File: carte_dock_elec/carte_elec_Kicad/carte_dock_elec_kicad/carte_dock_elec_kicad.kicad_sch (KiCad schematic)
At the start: 13 parts, among them J1 1758018, J10 Conn_02x20_Odd_Even, J2 22053021, J3 22272041, J4 22272041, J5 22272041, J6 1758018, J7 1758018, J8 1758018, J9 1758018, Q1 IRLB8748PBF

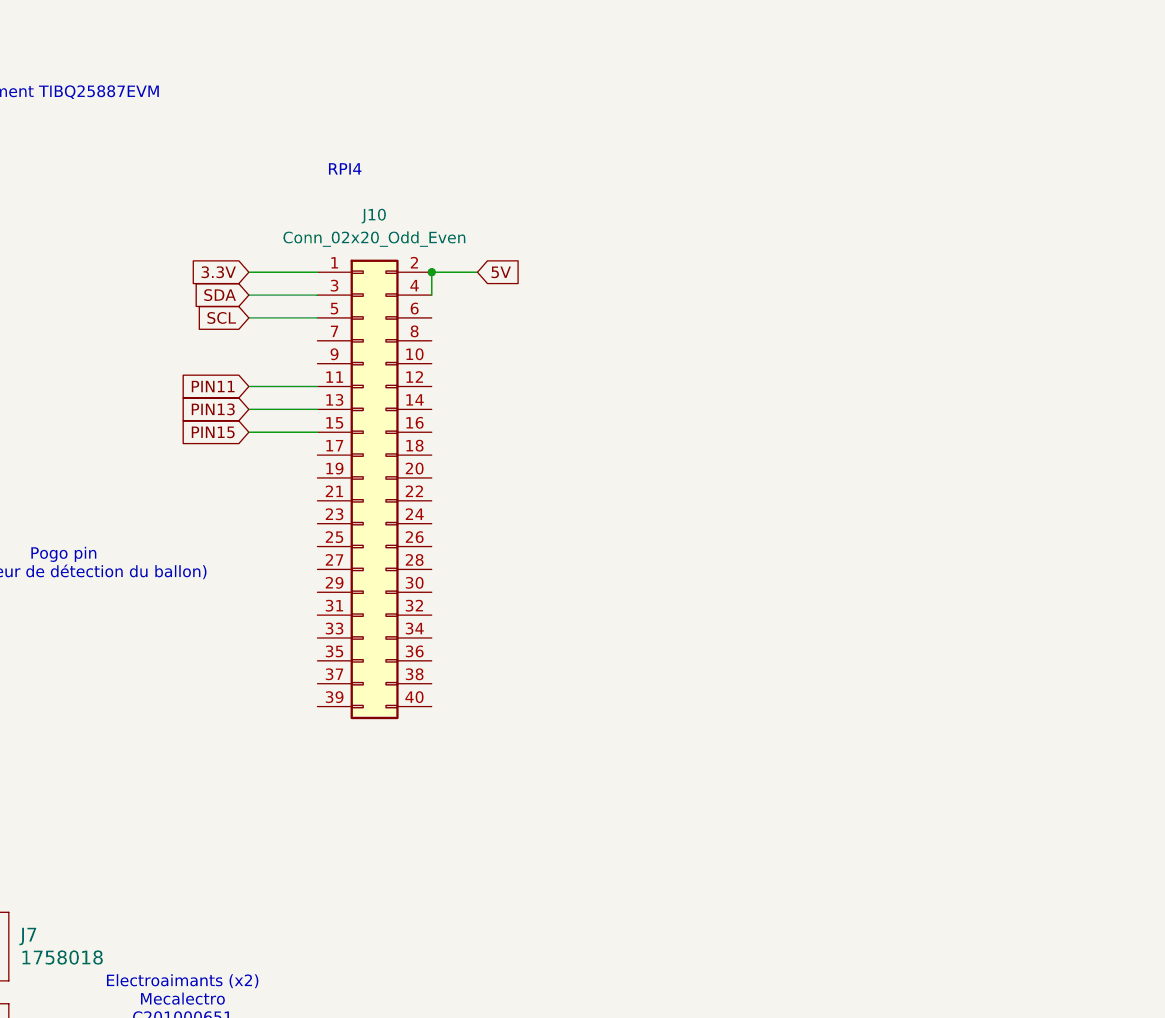
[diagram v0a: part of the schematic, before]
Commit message: carte_dock
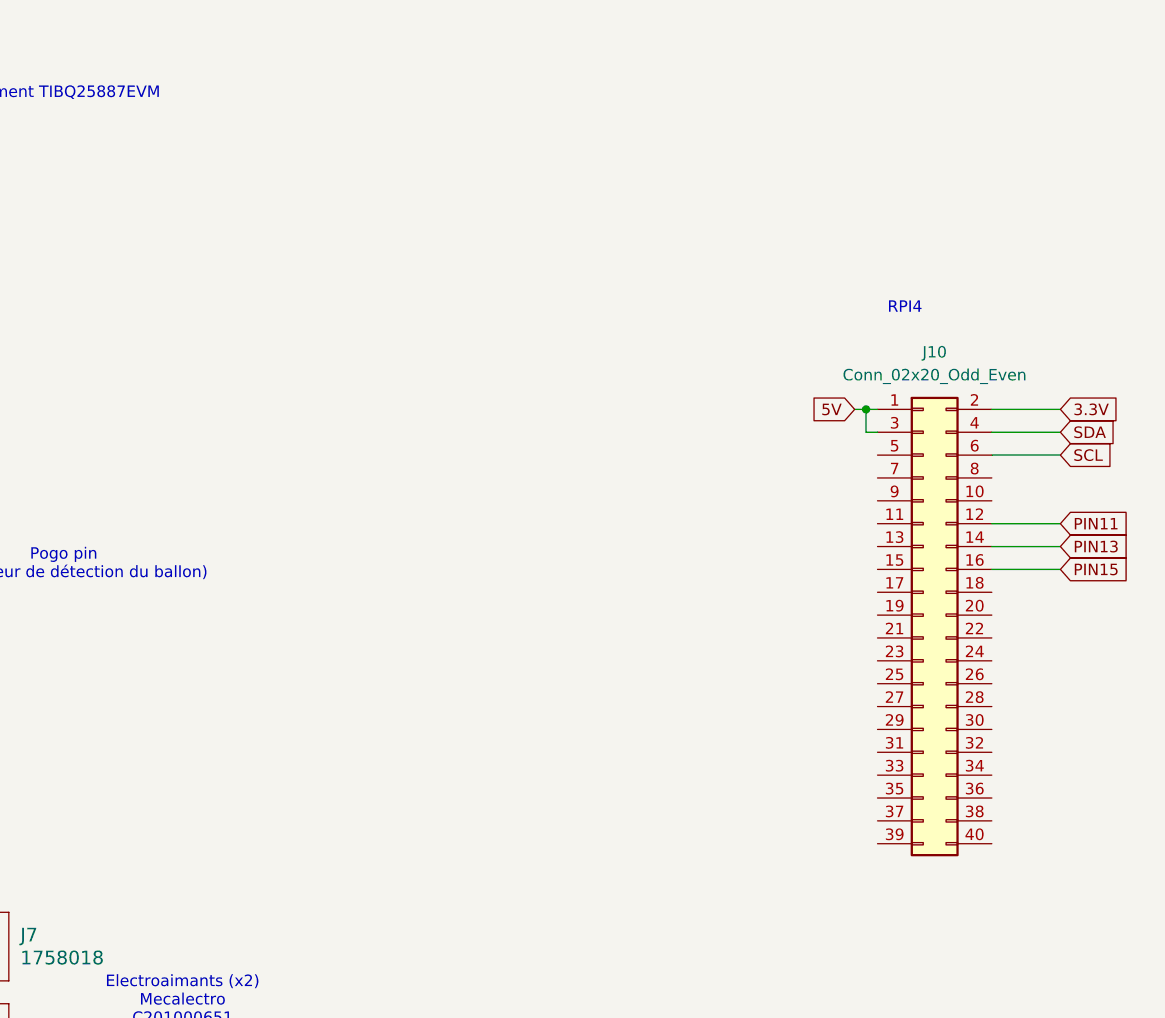
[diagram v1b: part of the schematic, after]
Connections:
- net 3.3V: now also J10.2 (Pin_2); no longer J10.1 (Pin_1)
- net 5V: now also J10.1 (Pin_1), J10.3 (Pin_3); no longer J10.2 (Pin_2), J10.4 (Pin_4)
- net PIN11: now also J10.12 (Pin_12); no longer J10.11 (Pin_11)
- net PIN13: now also J10.14 (Pin_14); no longer J10.13 (Pin_13)
- net PIN15: now also J10.16 (Pin_16); no longer J10.15 (Pin_15)
- net SCL: now also J10.6 (Pin_6); no longer J10.5 (Pin_5)
- net SDA: now also J10.4 (Pin_4); no longer J10.3 (Pin_3)
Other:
- moved on the sheet: J10

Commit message: MAJ DOCK ELEC
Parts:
- D1: footprint Diode_SMD:D_0201_0603Metric -> Diode_SMD:D_1206_3216Metric
- R1: footprint Resistor_SMD:R_0201_0603Metric -> Resistor_SMD:R_1206_3216Metric
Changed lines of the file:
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@@
 			)
 		)
-		(property "Footprint" "Diode_SMD:D_0201_0603Metric"
+		(property "Footprint" "Diode_SMD:D_1206_3216Metric"
 			(at 97.79 123.19 0)
 			(hide yes)
@@
 			)
 		)
-		(property "Footprint" "Resistor_SMD:R_0201_0603Metric"
+		(property "Footprint" "Resistor_SMD:R_1206_3216Metric"
 			(at 80.01 80.518 90)
 			(hide yes)
